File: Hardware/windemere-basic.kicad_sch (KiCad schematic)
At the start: 55 parts, among them J1 A_40-LC-TT, J2 A_40-LC-TT, J3 Connector, J4 A_28-LC-TT, J5 A_28-LC-TT, J6 Barrel_Jack, SW1 Reset Button, U1 MCP102-475, U2 HD44780U, U3 WD65C02, U4 28C256, U5 62256, U6 WD65C22, U7 74LS00, U8 MM74C923, U9 L7805, X1 1MHz

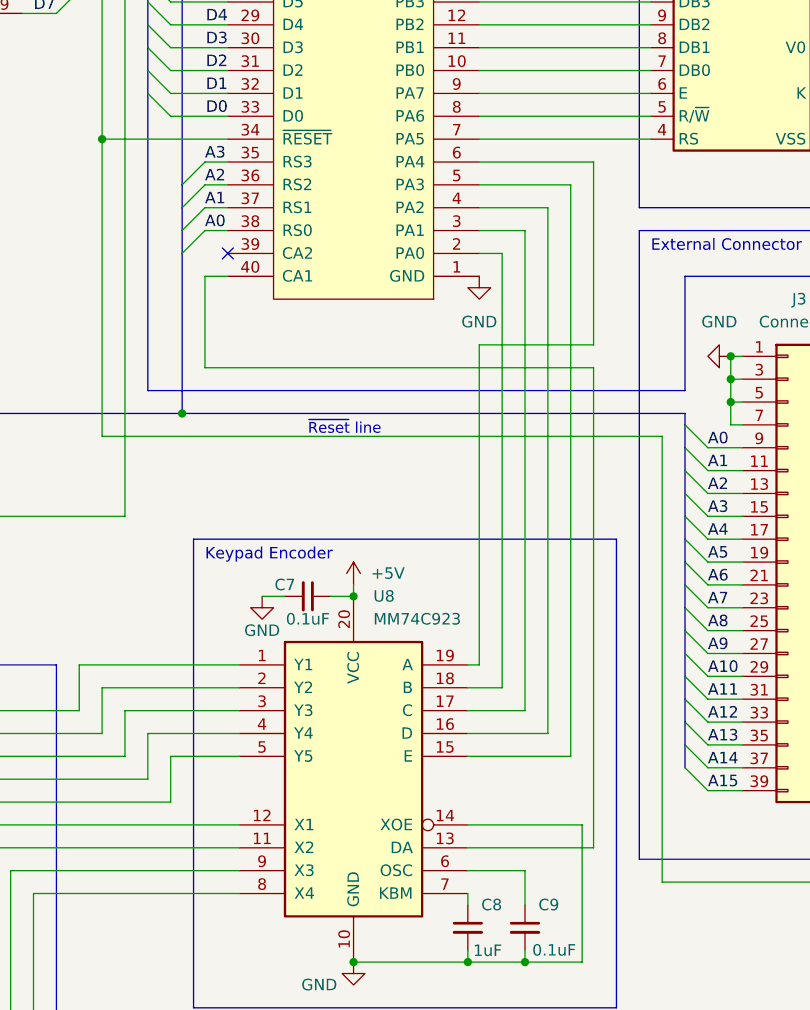
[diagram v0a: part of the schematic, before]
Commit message: Update windemere-basic.kicad_sch
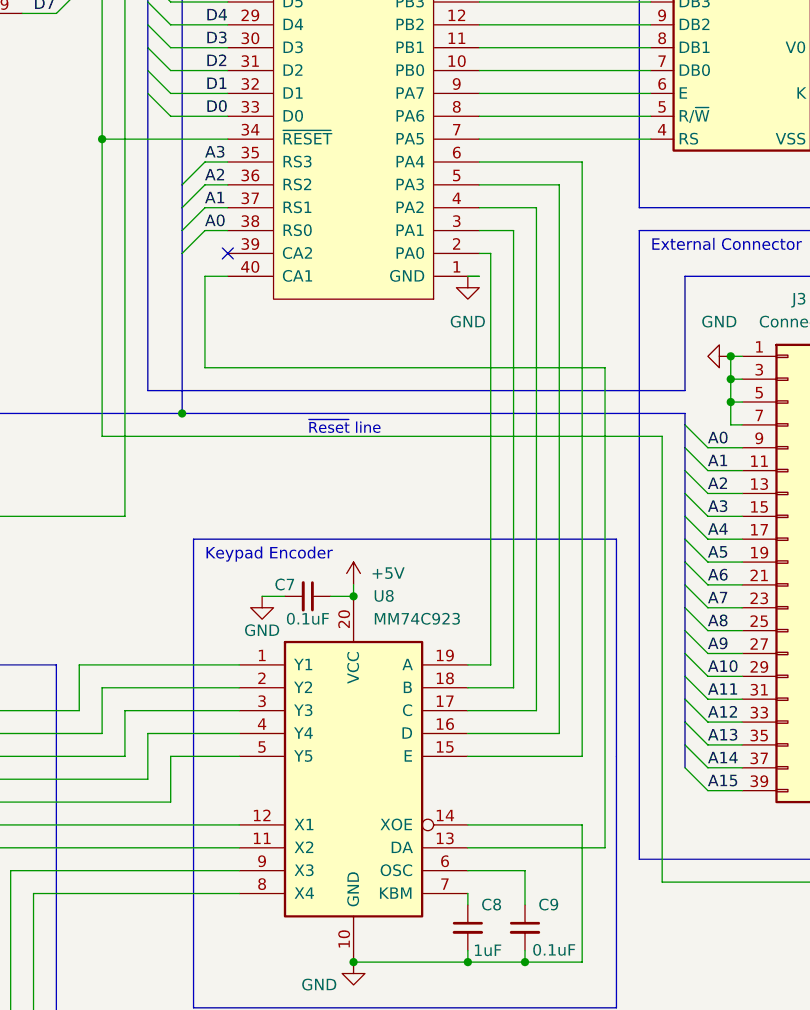
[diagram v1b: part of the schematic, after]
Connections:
- net at U6.2 (PA0): now also U8.19 (A); no longer U8.18 (B)
- net at U6.3 (PA1): now also U8.18 (B); no longer U8.17 (C)
- net at U6.4 (PA2): now also U8.17 (C); no longer U8.16 (D)
- net at U6.5 (PA3): now also U8.16 (D); no longer U8.15 (E)
- net at U6.6 (PA4): now also U8.15 (E); no longer U8.19 (A)
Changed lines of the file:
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@@
     (stroke (width 0) (type default))
   )
-  (wire (pts (xy 203.2 82.55) (xy 215.9 82.55))
+  (wire (pts (xy 201.93 138.43) (xy 204.47 138.43))
     (stroke (width 0) (type default))
   )
@@
     (stroke (width 0) (type default))
   )
-  (wire (pts (xy 172.72 105.41) (xy 215.9 105.41))
+  (wire (pts (xy 201.93 146.05) (xy 212.09 146.05))
+    (stroke (width 0) (type default))
+  )
+  (wire (pts (xy 172.72 105.41) (xy 217.17 105.41))
     (stroke (width 0) (type default))
   )
@@
     (stroke (width 0) (type default))
   )
+  (wire (pts (xy 214.63 82.55) (xy 203.2 82.55))
+    (stroke (width 0) (type default))
+  )
   (wire (pts (xy 168.91 74.93) (xy 175.26 74.93))
     (stroke (width 0) (type default))
@@
     (stroke (width 0) (type default))
   )
-  (wire (pts (xy 215.9 102.87) (xy 203.2 102.87))
-    (stroke (width 0) (type default))
-  )
   (wire (pts (xy 25.4 121.92) (xy 45.72 121.92))
     (stroke (width 0) (type default))
@@
     (stroke (width 0) (type default))
   )
+  (wire (pts (xy 209.55 143.51) (xy 209.55 87.63))
+    (stroke (width 0) (type default))
+  )
   (wire (pts (xy 50.8 161.29) (xy 57.15 161.29))
     (stroke (width 0) (type default))
@@
     (stroke (width 0) (type default))
   )
-  (wire (pts (xy 203.2 85.09) (xy 213.36 85.09))
-    (stroke (width 0) (type default))
-  )
   (wire (pts (xy 245.11 119.38) (xy 247.65 119.38))
     (stroke (width 0) (type default))
   )
+  (wire (pts (xy 207.01 140.97) (xy 207.01 90.17))
+    (stroke (width 0) (type default))
+  )
   (wire (pts (xy 88.9 124.46) (xy 88.9 129.54))
     (stroke (width 0) (type default))
@@
     (stroke (width 0) (type default))
   )
-  (wire (pts (xy 203.2 90.17) (xy 208.28 90.17))
-    (stroke (width 0) (type default))
-  )
   (wire (pts (xy 228.6 114.3) (xy 232.41 114.3))
     (stroke (width 0) (type default))
@@
     (stroke (width 0) (type default))
   )
+  (wire (pts (xy 214.63 148.59) (xy 214.63 82.55))
+    (stroke (width 0) (type default))
+  )
+  (wire (pts (xy 201.93 148.59) (xy 214.63 148.59))
+    (stroke (width 0) (type default))
+  )
   (wire (pts (xy 78.74 68.58) (xy 82.55 68.58))
     (stroke (width 0) (type default))
@@
     (stroke (width 0) (type default))
   )
+  (wire (pts (xy 201.93 143.51) (xy 209.55 143.51))
+    (stroke (width 0) (type default))
+  )
   (wire (pts (xy 106.68 156.21) (xy 106.68 168.91))
     (stroke (width 0) (type default))
@@
     (stroke (width 0) (type default))
   )
-  (wire (pts (xy 213.36 85.09) (xy 213.36 148.59))
-    (stroke (width 0) (type default))
-  )
   (wire (pts (xy 168.91 67.31) (xy 175.26 67.31))
     (stroke (width 0) (type default))
@@
     (stroke (width 0) (type default))
   )
+  (wire (pts (xy 212.09 85.09) (xy 203.2 85.09))
+    (stroke (width 0) (type default))
+  )
   (wire (pts (xy 115.57 107.95) (xy 115.57 26.67))
     (stroke (width 0) (type default))
@@
     (stroke (width 0) (type default))
   )
-  (wire (pts (xy 203.2 92.71) (xy 205.74 92.71))
-    (stroke (width 0) (type default))
-  )
   (wire (pts (xy 137.16 173.99) (xy 148.59 173.99))
     (stroke (width 0) (type default))
@@
     (stroke (width 0) (type default))
   )
-  (wire (pts (xy 208.28 90.17) (xy 208.28 143.51))
-    (stroke (width 0) (type default))
-  )
   (wire (pts (xy 245.11 109.22) (xy 246.38 109.22))
     (stroke (width 0) (type default))
@@
     (stroke (width 0) (type default))
   )
-  (wire (pts (xy 215.9 105.41) (xy 215.9 158.75))
-    (stroke (width 0) (type default))
-  )
-  (wire (pts (xy 205.74 92.71) (xy 205.74 140.97))
+  (wire (pts (xy 217.17 105.41) (xy 217.17 158.75))
     (stroke (width 0) (type default))
   )
@@
     (stroke (width 0) (type default))
   )
-  (wire (pts (xy 201.93 146.05) (xy 210.82 146.05))
-    (stroke (width 0) (type default))
-  )
   (wire (pts (xy 201.93 171.45) (xy 201.93 170.18))
     (stroke (width 0) (type default))
@@
     (stroke (width 0) (type default))
   )
-  (wire (pts (xy 210.82 87.63) (xy 210.82 146.05))
-    (stroke (width 0) (type default))
-  )
   (wire (pts (xy 173.99 46.99) (xy 175.26 46.99))
     (stroke (width 0) (type default))
@@
     (stroke (width 0) (type default))
   )
+  (wire (pts (xy 201.93 95.25) (xy 203.2 95.25))
+    (stroke (width 0) (type default))
+  )
   (wire (pts (xy 101.6 161.29) (xy 110.49 161.29))
     (stroke (width 0) (type default))
   )
-  (wire (pts (xy 201.93 148.59) (xy 213.36 148.59))
-    (stroke (width 0) (type default))
-  )
   (wire (pts (xy 78.74 53.34) (xy 82.55 53.34))
     (stroke (width 0) (type default))
@@
     (stroke (width 0) (type default))
   )
+  (wire (pts (xy 204.47 92.71) (xy 203.2 92.71))
+    (stroke (width 0) (type default))
+  )
   (wire (pts (xy 123.19 73.66) (xy 127 73.66))
     (stroke (width 0) (type default))
@@
     (stroke (width 0) (type default))
   )
-  (wire (pts (xy 208.28 143.51) (xy 201.93 143.51))
-    (stroke (width 0) (type default))
-  )
   (wire (pts (xy 171.45 57.15) (xy 175.26 57.15))
     (stroke (width 0) (type default))
@@
     (stroke (width 0) (type default))
   )
+  (wire (pts (xy 201.93 140.97) (xy 207.01 140.97))
+    (stroke (width 0) (type default))
+  )
   (wire (pts (xy 203.2 74.93) (xy 222.25 74.93))
     (stroke (width 0) (type default))
@@
     (stroke (width 0) (type default))
   )
+  (wire (pts (xy 204.47 138.43) (xy 204.47 92.71))
+    (stroke (width 0) (type default))
+  )
   (wire (pts (xy 234.95 27.94) (xy 234.95 29.21))
     (stroke (width 0) (type default))
@@
     (stroke (width 0) (type default))
   )
-  (wire (pts (xy 205.74 140.97) (xy 201.93 140.97))
-    (stroke (width 0) (type default))
-  )
   (wire (pts (xy 172.72 82.55) (xy 175.26 82.55))
     (stroke (width 0) (type default))
@@
     (stroke (width 0) (type default))
   )
-  (wire (pts (xy 201.93 158.75) (xy 215.9 158.75))
+  (wire (pts (xy 201.93 158.75) (xy 217.17 158.75))
     (stroke (width 0) (type default))
   )
@@
     (stroke (width 0) (type default))
   )
-  (wire (pts (xy 201.93 138.43) (xy 203.2 138.43))
-    (stroke (width 0) (type default))
-  )
   (wire (pts (xy 189.23 24.13) (xy 209.55 24.13))
     (stroke (width 0) (type default))
@@
     (stroke (width 0) (type default))
   )
-  (wire (pts (xy 203.2 87.63) (xy 210.82 87.63))
-    (stroke (width 0) (type default))
-  )
   (wire (pts (xy 245.11 116.84) (xy 247.65 116.84))
     (stroke (width 0) (type default))
@@
     (stroke (width 0) (type default))
   )
+  (wire (pts (xy 207.01 90.17) (xy 203.2 90.17))
+    (stroke (width 0) (type default))
+  )
   (wire (pts (xy 63.5 86.36) (xy 73.66 86.36))
     (stroke (width 0) (type default))
@@
     (stroke (width 0) (type default))
   )
+  (wire (pts (xy 209.55 87.63) (xy 203.2 87.63))
+    (stroke (width 0) (type default))
+  )
   (polyline (pts (xy 265.43 132.08) (xy 252.73 132.08))
     (stroke (width 0) (type default))
@@
     (stroke (width 0) (type default))
   )
+  (wire (pts (xy 212.09 146.05) (xy 212.09 85.09))
+    (stroke (width 0) (type default))
+  )
   (wire (pts (xy 66.04 26.67) (xy 66.04 55.88))
     (stroke (width 0) (type default))
@@
   )
   (wire (pts (xy 227.33 27.94) (xy 234.95 27.94))
-    (stroke (width 0) (type default))
-  )
-  (wire (pts (xy 203.2 102.87) (xy 203.2 138.43))
-    (stroke (width 0) (type default))
-  )
-  (wire (pts (xy 215.9 82.55) (xy 215.9 102.87))
     (stroke (width 0) (type default))
   )
@@
     )
   )
-  (symbol (lib_id "power:GND") (at 203.2 95.25 0) (unit 1)
+  (symbol (lib_id "power:GND") (at 201.93 95.25 0) (unit 1)
     (in_bom yes) (on_board yes) (dnp no) (fields_autoplaced)
-    (property "Reference" "#PWR020" (at 203.2 101.6 0)
-      (effects (font (size 1.27 1.27)) hide)
-    )
-    (property "Value" "GND" (at 203.2 100.33 0)
+    (property "Reference" "#PWR020" (at 201.93 101.6 0)
+      (effects (font (size 1.27 1.27)) hide)
+    )
+    (property "Value" "GND" (at 201.93 100.33 0)
       (effects (font (size 1.27 1.27)))
     )
-    (property "Footprint" "" (at 203.2 95.25 0)
-      (effects (font (size 1.27 1.27)) hide)
-    )
-    (property "Datasheet" "" (at 203.2 95.25 0)
-      (effects (font (size 1.27 1.27)) hide)
-    )
+    (property "Footprint" "" (at 201.93 95.25 0)
+      (effects (font (size 1.27 1.27)) hide)
+    )
+    (property "Datasheet" "" (at 201.93 95.25 0)
+      (effects (font (size 1.27 1.27)) hide)
+    )

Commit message: Correct MM74C923
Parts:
- J3: footprint Connector_PCBEdge:Samtec_MECF-20-0_-NP-L-DV_2x20_P1.27mm_Edge -> Connector_PinHeader_2.54mm:PinHeader_2x20_P2.54mm_Vertical
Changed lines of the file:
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@@
       (effects (font (size 1.27 1.27)))
     )
-    (property "Footprint" "Connector_PCBEdge:Samtec_MECF-20-0_-NP-L-DV_2x20_P1.27mm_Edge" (at 237.49 127 0)
+    (property "Footprint" "Connector_PinHeader_2.54mm:PinHeader_2x20_P2.54mm_Vertical" (at 237.49 127 0)
       (effects (font (size 1.27 1.27)) hide)
     )
